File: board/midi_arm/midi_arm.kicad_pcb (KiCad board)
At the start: 2 copper layers, 100 x 100 mm, 24 parts, among them J2 Conn_01x03_Pin, J3 Conn_01x04_Pin, J4 Conn_01x05_Pin, SW1 SW_MEC_5E, SW2 SW_DIP_x01

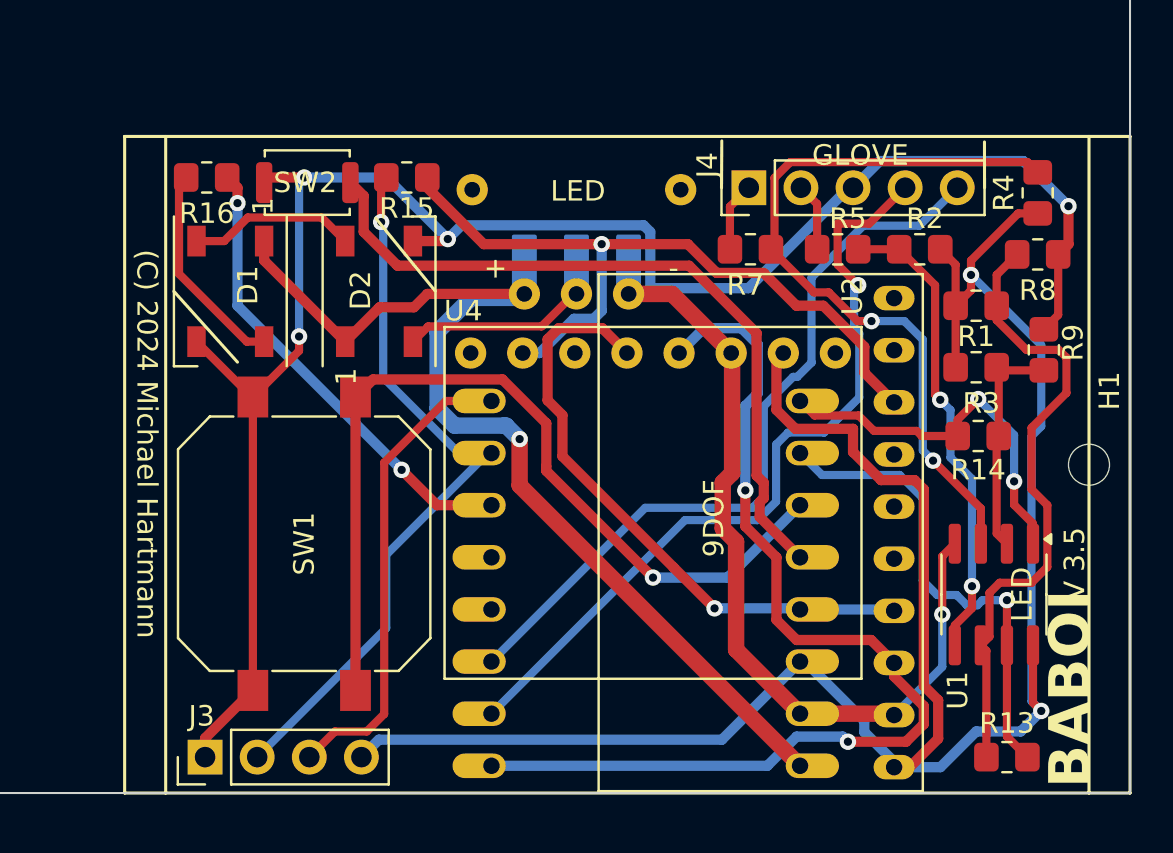
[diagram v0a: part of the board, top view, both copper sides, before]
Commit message: rev 4 board
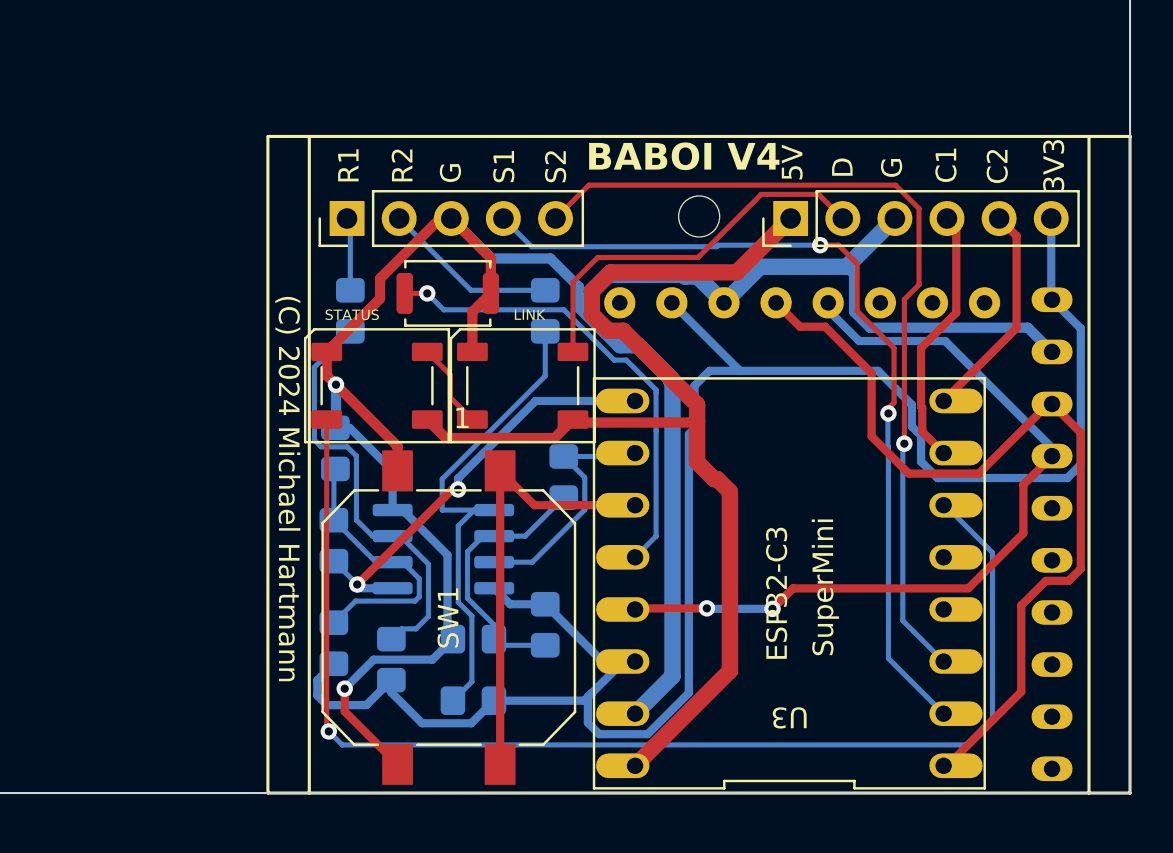
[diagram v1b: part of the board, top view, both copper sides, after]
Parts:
- removed J2: Conn_01x03_Pin, midi_arm:LED_conn
- removed J3: Conn_01x04_Pin, Connector_PinHeader_2.54mm:PinHeader_1x04_P2.54mm_Vertical
- removed R15: 0k, Resistor_SMD:R_0805_2012Metric_Pad1.20x1.40mm_HandSolder
- removed R16: 24K, Resistor_SMD:R_0805_2012Metric_Pad1.20x1.40mm_HandSolder
- added J1: Conn_01x06_Socket, Connector_PinHeader_2.54mm:PinHeader_1x06_P2.54mm_Vertical, F.Cu at (173.5, 97.0)
- R1, R13, R14, R2, R3, R4, R5, R7, R8, R9, U1, U2, U4: moved to B.Cu
- U3: moved to F.Cu
- moved R4 38.9 mm to (154.0, 118.5)
- moved R9 34.9 mm to (151.3, 108.2)
- moved R3 34.1 mm to (151.2, 117.7), turned to 90 degrees
- moved R8 33.3 mm to (158.0, 117.5), turned to 180 degrees
- moved R14 31.8 mm to (151.2, 112.7), turned to -90 degrees
- moved R2 30.9 mm to (158.0, 120.5)
- moved U1 26.9 mm to (156.5, 113.1), turned to 0 degrees
- moved R1 26.1 mm to (161.5, 116.8), turned to -90 degrees
- moved R13 25.6 mm to (162.4, 109.6), turned to 90 degrees
- moved H1 22.5 mm to (169.0, 96.9)
- moved U4 20.8 mm to (160.1, 101.1)
- moved R7 19.7 mm to (152.0, 101.5), turned to -90 degrees
- moved J4 19.6 mm to (151.8, 97.0)
- moved R5 14.6 mm to (161.5, 101.5), turned to -90 degrees
- moved SW2 8.72 mm to (156.8, 100.7), turned to 0 degrees
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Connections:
- U2 pad 8: Net-(U2-INT) -> unconnected-(U2-INT-Pad8)
- U3 pad 14: Net-(U3-GPIO10) -> Net-(D1-DIN)
- U4 pad 7: Net-(U2-INT) -> unconnected-(U4-A_INT1-Pad7)
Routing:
- net Net-(D1-DIN): track 10.4 -> 59.7 mm, vias 0 -> 1
- net Net-(U2-INT): track 35.8 -> 0.00 mm, vias 1 -> 0
- net Net-(J1-Pin_4): track 36.3 -> 12.1 mm, vias 1 -> 0
- net Net-(U3-GPIO10): track 22.9 -> 0.00 mm, vias 2 -> 0
- net /BUTTON1: track 43.4 -> 21.6 mm, vias 1 -> 0
- net Net-(U1-VinB-): track 30.6 -> 12.2 mm
- net Net-(U1-VinA+): track 37.2 -> 20.3 mm, vias 2 -> 0
- net GND1: track 130.1 -> 113.9 mm, vias 5 -> 2
- net /VCC_3V3: track 105.5 -> 89.5 mm, vias 2 -> 0
- net /BUTTON2: track 35.8 -> 22.8 mm, vias 0 -> 1
- net Net-(J1-Pin_5): track 23.2 -> 10.7 mm
- net /ADC1_1: track 24.3 -> 11.8 mm, vias 1 -> 0
- net Net-(D2-DOUT): track 8.93 -> 18.8 mm
- net /SCL: track 51.3 -> 41.8 mm, vias 2 -> 0
- net /SDA: track 30.0 -> 39.3 mm, vias 1 -> 2
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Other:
- board text added: "3V3"
- board text added: "5V"
- board text added: "BABOI V4"
- board text added: "C1"
- board text added: "C2"
- board text added: "D"
- board text added: "G"
- board text added: "LINK"
- board text added: "R1"
- board text added: "R2"
- board text added: "S1"
- board text added: "S2"
- board text added: "STATUS"
- board text removed: "+"
- board text removed: "-"
- board text removed: "BABOI"
- board text removed: "GLOVE"
- board text removed: "LED"
- board text removed: "V 3.5"
